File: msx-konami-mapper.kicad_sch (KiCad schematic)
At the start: 10 parts, among them SW1 Bonus Games, U1 SST39SF040, U3 74LS670, U4 74LS02

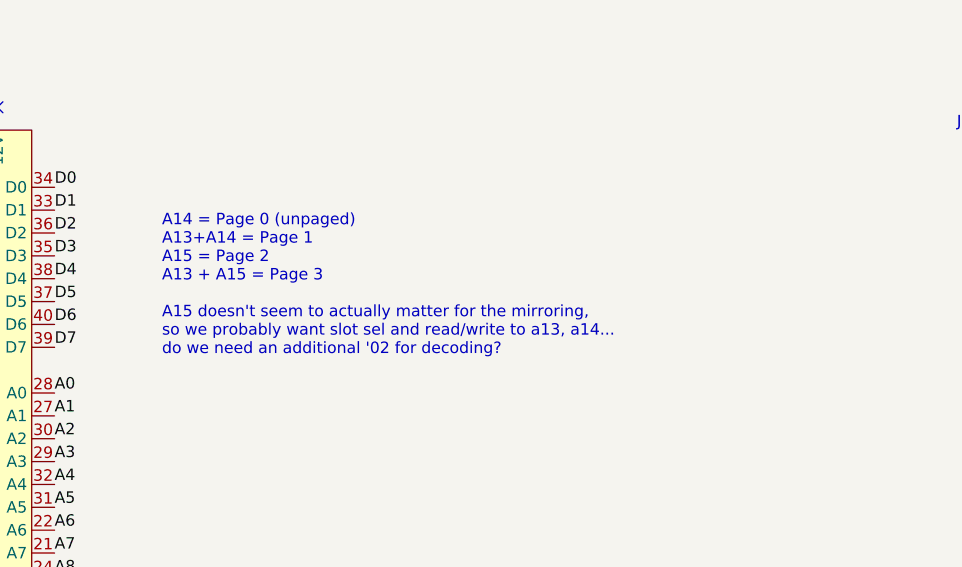
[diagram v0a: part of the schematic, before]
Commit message: Better explainer
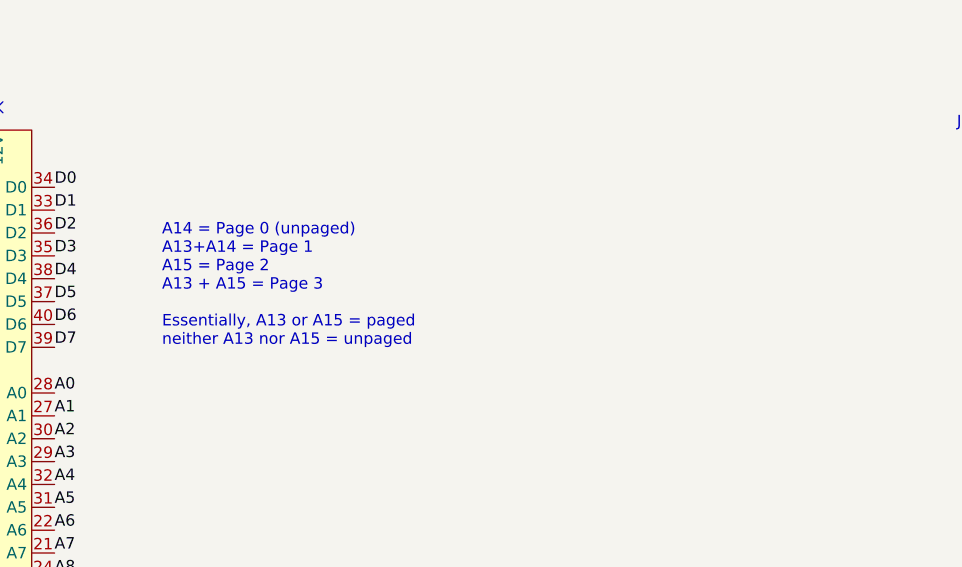
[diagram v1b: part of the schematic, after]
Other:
- note added: "A14 = Page 0 (unpaged) A13+A14 = Page 1 A15 = Page 2 A13 + A15 = Page 3 Essentially, A13 or A15 = paged neither A13 nor A15 = unpaged"
- note removed: "A14 = Page 0 (unpaged) A13+A14 = Page 1 A15 = Page 2 A13 + A15 = Page 3 A15 doesn't seem to actually matter for the mirroring, so we probably want slot sel and read/write to a13, a14... do we need an additional '02 for decoding?"
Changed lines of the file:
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@@
 		)
 	)
-	(text "A14 = Page 0 (unpaged)\nA13+A14 = Page 1\nA15 = Page 2\nA13 + A15 = Page 3\n\nA15 doesn't seem to actually matter for the mirroring,\nso we probably want slot sel and read/write to a13, a14...\ndo we need an additional '02 for decoding?"
+	(text "A14 = Page 0 (unpaged)\nA13+A14 = Page 1\nA15 = Page 2\nA13 + A15 = Page 3\n\nEssentially, A13 or A15 = paged\nneither A13 nor A15 = unpaged"
 		(exclude_from_sim no)
 		(at 71.628 90.932 0)

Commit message: Prepare for BOM release
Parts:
- U2: now left out of the parts list
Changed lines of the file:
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@@
 		(unit 1)
 		(exclude_from_sim no)
-		(in_bom yes)
+		(in_bom no)
 		(on_board yes)
 		(dnp no)

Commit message: DK part numbers
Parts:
- C2, C3: DigiKey (none) -> 399-9776-ND
- RN1: DigiKey (none) -> 4609X-101-103LF-ND
- U1: DigiKey (none) -> SST39SF040-70-4C-PHE-ND
- U3: DigiKey (none) -> 296-34025-5-ND
- U4: DigiKey (none) -> 296-1627-5-ND
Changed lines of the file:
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@@
+			)
+		)
+		(property "DigiKey" "399-9776-ND"
+			(at 210.82 142.24 0)
+			(effects
+				(font
+					(size 1.27 1.27)
+				)
+				(hide yes)
 			)
 		)
@@
 			)
 		)
+		(property "DigiKey" "296-1627-5-ND"
+			(at 95.25 44.45 0)
+			(effects
+				(font
+					(size 1.27 1.27)
+				)
+				(hide yes)
+			)
+		)
 		(pin "7"
 		)
@@
 		)
 		(property "Description" "quad 2-input NOR gate"
+			(at 95.25 27.94 0)
+			(effects
+				(font
+					(size 1.27 1.27)
+				)
+				(hide yes)
+			)
+		)
+		(property "DigiKey" "296-1627-5-ND"
 			(at 95.25 27.94 0)
 			(effects
@@
 			)
 		)
+		(property "DigiKey" "296-1627-5-ND"
+			(at 154.94 175.26 0)
+			(effects
+				(font
+					(size 1.27 1.27)
+				)
+				(hide yes)
+			)
+		)
 		(pin "2"
 		)
@@
 			)
 		)
+		(property "DigiKey" "399-9776-ND"
+			(at 224.79 142.24 0)
+			(effects
+				(font
+					(size 1.27 1.27)
+				)
+				(hide yes)
+			)
+		)
 		(pin "1"
 		)
@@
 			)
 		)
+		(property "DigiKey" "296-34025-5-ND"
+			(at 191.77 41.91 0)
+			(effects
+				(font
+					(size 1.27 1.27)
+				)
+				(hide yes)
+			)
+		)
 		(pin "1"
 		)
@@
 			)
 		)
+		(property "DigiKey" "SST39SF040-70-4C-PHE-ND"
+			(at 264.16 69.85 0)
+			(effects
+				(font
+					(size 1.27 1.27)
+				)
+				(hide yes)
+			)
+		)
 		(pin "19"
 		)
@@
 		)
 		(property "Description" "8 resistor network, star topology, bussed resistors, small US symbol"
+			(at 223.52 44.45 0)
+			(effects
+				(font
+					(size 1.27 1.27)
+				)
+				(hide yes)
+			)
+		)
+		(property "DigiKey" "4609X-101-103LF-ND"
 			(at 223.52 44.45 0)
 			(effects
@@
 			)
 		)
+		(property "DigiKey" "296-1627-5-ND"
+			(at 138.43 177.8 0)
+			(effects
+				(font
+					(size 1.27 1.27)
+				)
+				(hide yes)
+			)
+		)
 		(pin "2"
 		)
@@
 			(at 111.76 27.94 0)
 			(effects
+				(font
+					(size 1.27 1.27)
+				)
+				(hide yes)
+			)
+		)
+		(property "DigiKey" "296-1627-5-ND"
+			(at 111.76 27.94 0)
+			(effects
